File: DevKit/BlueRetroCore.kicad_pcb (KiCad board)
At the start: 4 copper layers, 85 x 56 mm, 108 parts, among them J1 USB_C_Receptacle_USB2.0, J2 Conn_02x06, J3 Micro_SD_Card, J4 Conn_01x03, J5 DB25_Female_MountingHoles, J6 Conn_02x13, J7 Conn_02x07, Q1 BSS138, Q2 BSS138, Q3 S8050, Q4 S8050, Q5 S8050, SW1 BOOT, SW2 EN, U1 ESP32-WROOM, U10 TPD6F003, U11 TPD6F003, U12 TPD6F003, U13 TPD6F003, U2 FT2232HL, U3 STL6N3LLH6, U4 TCPP01-M12, U5 M93C46, U6 ECMF02-2AMX6, U7 TPD6F003, U8 AP7361C-33E, U9 AP7361C-33E, Y1 12MHz

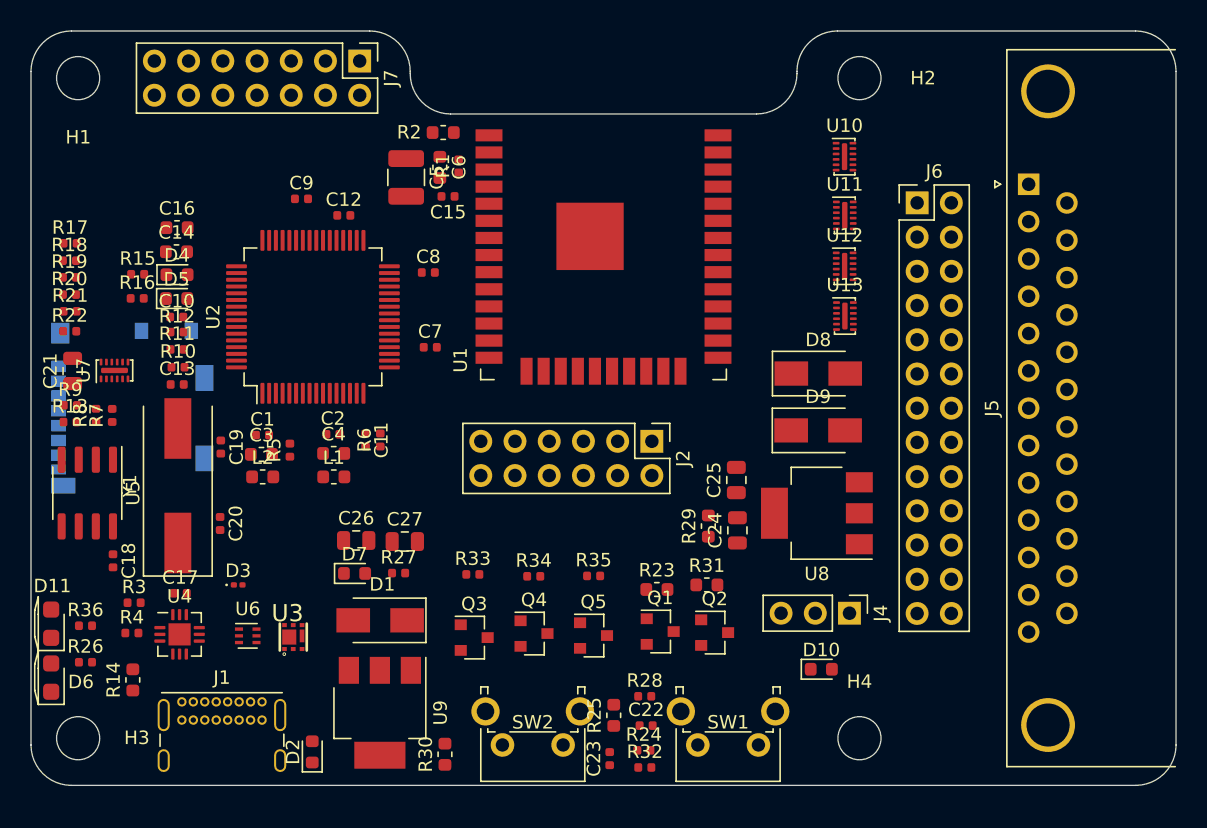
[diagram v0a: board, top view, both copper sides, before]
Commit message: PCB routing
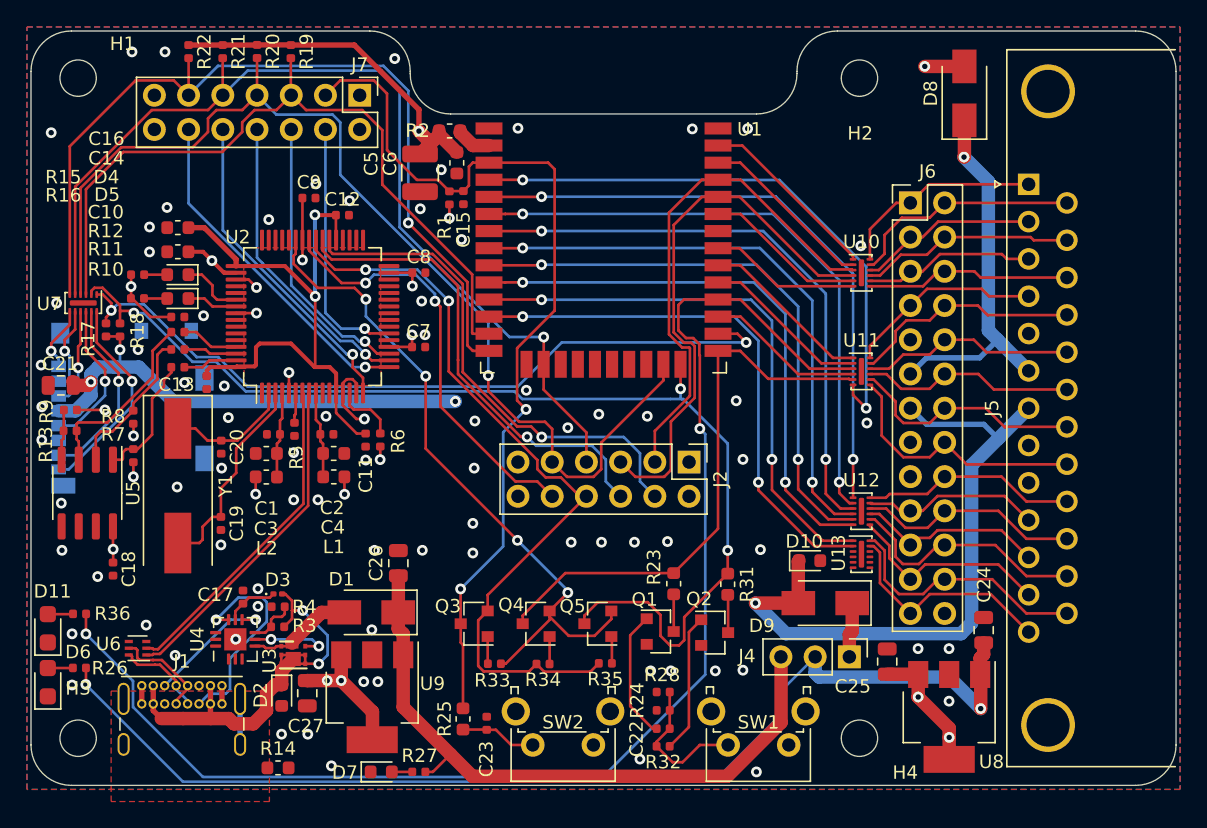
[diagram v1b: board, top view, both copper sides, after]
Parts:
- removed R29, R30: 0, BlueRetro:R_0603_1608Metric
- H1, H2, H3, H4: footprint BlueRetro:MountingHole_3.2mm_M3 -> BlueRetro:MountingHole_2.7mm_M2.5
- U1: value ESP32-WROOM -> ESP32-WROOM-32E
- U8, U9: footprint BlueRetro:SOT-223-3_TabPin2 -> BlueRetro:SOT-223-3_TabPin3
- moved R19 23.5 mm to (-23.2, -26.5), turned to 270 degrees
- moved D8 23.5 mm to (26.8, -23.4), turned to 90 degrees
- moved R20 22.8 mm to (-25.7, -26.5), turned to 270 degrees
- moved R22 22.6 mm to (-30.8, -26.5), turned to 270 degrees
- moved R21 22.4 mm to (-28.3, -26.5), turned to 270 degrees
- moved C24 19.7 mm to (28.2, 16.5)
- moved U12 18.2 mm to (19.1, 7.65)
- moved U8 18.0 mm to (25.7, 22.9), turned to 270 degrees
- moved U13 17.7 mm to (19.1, 10.8)
- moved C25 17.5 mm to (21.1, 18.8)
- moved D7 14.9 mm to (-16.5, 27.0)
- moved R27 14.8 mm to (-13.7, 27.0), turned to 180 degrees
- moved C27 13.4 mm to (-22.0, 21.2), turned to 270 degrees
- moved D9 12.8 mm to (16.5, 14.5), turned to 180 degrees
- moved R14 12.6 mm to (-24.2, 26.7), turned to 0 degrees
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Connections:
- net Net-(J1-PadA6) renamed /USB_C_P
- net Net-(J1-PadA7) renamed /USB_C_N
- net Net-(U2-Pad7) renamed /USB_N
- net Net-(U2-Pad8) renamed /USB_P
- J1 pad A8: (no net) -> Net-(J1-PadA8)
- J1 pad B8: (no net) -> Net-(J1-PadB8)
- J3 pad 10: (no net) -> Net-(J3-Pad10)
- J3 pad 9: (no net) -> Net-(J3-Pad9)
- J5 pad 1: /IO19_C -> /IO23_C
- J5 pad 10: /IO32_C -> /I34_C
- J5 pad 11: /IO33_C -> /IO32_C
- J5 pad 12: /I34_C -> /IO25_C
- J5 pad 13: /I35_C -> /IO27_C
- J5 pad 14: /IO0_C -> /IO22_C
- J5 pad 15: /IO1_C -> /IO3_C
- J5 pad 16: /IO3_C -> /IO19_C
- J5 pad 18: /IO16_C -> /IO17_C
- J5 pad 19: /IO17_C -> /IO16_C
- J5 pad 2: /IO21_C -> /IO1_C
- J5 pad 20: /IO18_C -> /IO0_C
- J5 pad 21: /IO23_C -> /I36_C
- J5 pad 22: /IO26_C -> /I39_C
- J5 pad 23: /IO27_C -> /I35_C
- J5 pad 24: /I36_C -> /IO33_C
- J5 pad 25: /I39_C -> /IO26_C
- J5 pad 3: /IO22_C -> /IO21_C
- J5 pad 4: /IO25_C -> /IO18_C
- J6 pad 1: /IO19_C -> /IO23_C
- J6 pad 10: /IO32_C -> /I34_C
- J6 pad 11: /IO33_C -> /IO32_C
- J6 pad 12: /I34_C -> /IO25_C
- J6 pad 13: /I35_C -> /IO27_C
- J6 pad 14: /IO0_C -> /IO22_C
- J6 pad 15: /IO1_C -> /IO3_C
- J6 pad 16: /IO3_C -> /IO19_C
- J6 pad 18: /IO16_C -> /IO17_C
- J6 pad 19: /IO17_C -> /IO16_C
- J6 pad 2: /IO21_C -> /IO1_C
- J6 pad 20: /IO18_C -> /IO0_C
- J6 pad 21: /IO23_C -> /I36_C
- J6 pad 22: /IO26_C -> /I39_C
- J6 pad 23: /IO27_C -> /I35_C
- J6 pad 24: /I36_C -> /IO33_C
- J6 pad 25: /I39_C -> /IO26_C
- J6 pad 3: /IO22_C -> /IO21_C
- J6 pad 4: /IO25_C -> /IO18_C
- J7 pad 10: /TMS -> /TCK
- J7 pad 11: /EN -> /IO12
- J7 pad 12: /nTRST -> /TDI
- J7 pad 3: /IO13 -> /EN
- J7 pad 4: /TCK -> /nTRST
- J7 pad 5: /IO12 -> /IO14
- J7 pad 6: /TDI -> /TMS
- J7 pad 9: /IO14 -> /IO13
- U1 pad 17: (no net) -> Net-(U1-Pad17)
- U1 pad 18: (no net) -> Net-(U1-Pad18)
- U1 pad 19: (no net) -> Net-(U1-Pad19)
- U1 pad 20: (no net) -> Net-(U1-Pad20)
- U1 pad 21: (no net) -> Net-(U1-Pad21)
- U1 pad 22: (no net) -> Net-(U1-Pad22)
- U1 pad 32: (no net) -> Net-(U1-Pad32)
- U10 pad 1: /IO19 -> /IO23
- U10 pad 10: /IO21_C -> /IO1_C
- U10 pad 11: /IO0_C -> /IO22_C
- U10 pad 12: /IO19_C -> /IO23_C
- U10 pad 2: /IO0 -> /IO22
- U10 pad 3: /IO21 -> /IO1
- U10 pad 4: /IO1 -> /IO3
- U10 pad 5: /IO22 -> /IO21
- U10 pad 6: /IO3 -> /IO19
- U10 pad 7: /IO3_C -> /IO19_C
- U10 pad 8: /IO22_C -> /IO21_C
- U10 pad 9: /IO1_C -> /IO3_C
- U11 pad 1: /IO25 -> /IO18
- U11 pad 10: /IO16_C -> /IO17_C
- U11 pad 12: /IO25_C -> /IO18_C
- U11 pad 3: /IO16 -> /IO17
- U11 pad 4: /IO17 -> /IO16
- U11 pad 5: /IO18 -> /IO0
- U11 pad 6: /IO23 -> /I36
- U11 pad 7: /IO23_C -> /I36_C
- U11 pad 8: /IO18_C -> /IO0_C
- U11 pad 9: /IO17_C -> /IO16_C
- U12 pad 1: /IO26 -> /I39
- U12 pad 10: /IO27_C -> /I35_C
- U12 pad 11: /IO32_C -> /I34_C
- U12 pad 12: /IO26_C -> /I39_C
- U12 pad 2: /IO32 -> /I34
- U12 pad 3: /IO27 -> /I35
- U12 pad 4: /IO33 -> /IO32
- U12 pad 5: /I36 -> /IO33
- U12 pad 6: /I34 -> /IO25
- U12 pad 7: /I34_C -> /IO25_C
- U12 pad 8: /I36_C -> /IO33_C
- U12 pad 9: /IO33_C -> /IO32_C
- U13 pad 1: /I39 -> /IO26
- U13 pad 10: (no net) -> Net-(U13-Pad10)
- U13 pad 11: /I35_C -> /IO27_C
- U13 pad 12: /I39_C -> /IO26_C
- U13 pad 2: /I35 -> /IO27
- U13 pad 3: (no net) -> Net-(U13-Pad3)
- U13 pad 4: (no net) -> Net-(U13-Pad4)
- U13 pad 5: (no net) -> Net-(U13-Pad5)
- U13 pad 6: (no net) -> Net-(U13-Pad6)
- U13 pad 7: (no net) -> Net-(U13-Pad7)
- U13 pad 8: (no net) -> Net-(U13-Pad8)
- U13 pad 9: (no net) -> Net-(U13-Pad9)
- U2 pad 21: (no net) -> Net-(U2-Pad21)
- U2 pad 23: (no net) -> Net-(U2-Pad23)
- U2 pad 24: (no net) -> Net-(U2-Pad24)
- U2 pad 26: (no net) -> Net-(U2-Pad26)
- U2 pad 27: (no net) -> Net-(U2-Pad27)
- U2 pad 28: (no net) -> Net-(U2-Pad28)
- U2 pad 29: (no net) -> Net-(U2-Pad29)
- U2 pad 30: (no net) -> Net-(U2-Pad30)
- U2 pad 32: (no net) -> Net-(U2-Pad32)
- U2 pad 33: (no net) -> Net-(U2-Pad33)
- U2 pad 34: (no net) -> Net-(U2-Pad34)
- U2 pad 36: (no net) -> Net-(U2-Pad36)
- U2 pad 44: (no net) -> Net-(U2-Pad44)
- U2 pad 45: (no net) -> Net-(U2-Pad45)
- U2 pad 46: (no net) -> Net-(U2-Pad46)
- U2 pad 48: (no net) -> Net-(U2-Pad48)
- U2 pad 52: (no net) -> Net-(U2-Pad52)
- U2 pad 53: (no net) -> Net-(U2-Pad53)
- U2 pad 57: (no net) -> Net-(U2-Pad57)
- U2 pad 58: (no net) -> Net-(U2-Pad58)
- U2 pad 59: (no net) -> Net-(U2-Pad59)
- U2 pad 60: (no net) -> Net-(U2-Pad60)
- U3 pad 1: Net-(D1-Pad2) -> Net-(D2-Pad1)
- U3 pad 2: Net-(D1-Pad2) -> Net-(D2-Pad1)
- U3 pad 3: Net-(D1-Pad2) -> Net-(U3-Pad3)
- U3 pad 4: Net-(U3-Pad4) -> Net-(D1-Pad2)
- U3 pad 8: Net-(D2-Pad1) -> Net-(D1-Pad2)
- U4 pad 5: Net-(U3-Pad4) -> Net-(U3-Pad3)
- U5 pad 6: (no net) -> Net-(U5-Pad6)
- U5 pad 7: (no net) -> Net-(U5-Pad7)
- U6 pad 4: (no net) -> Net-(U6-Pad4)
- U7 pad 1: /IO12 -> /IO4
- U7 pad 10: Net-(J3-Pad3) -> Net-(J3-Pad5)
- U7 pad 11: Net-(J3-Pad2) -> Net-(J3-Pad7)
- U7 pad 12: Net-(J3-Pad1) -> Net-(J3-Pad8)
- U7 pad 2: /IO13 -> /IO2
- U7 pad 3: /IO15 -> /IO14
- U7 pad 4: /IO14 -> /IO15
- U7 pad 5: /IO2 -> /IO13
- U7 pad 6: /IO4 -> /IO12
- U7 pad 7: Net-(J3-Pad8) -> Net-(J3-Pad1)
- U7 pad 8: Net-(J3-Pad7) -> Net-(J3-Pad2)
- U7 pad 9: Net-(J3-Pad5) -> Net-(J3-Pad3)
- U8 pad 2: Net-(R29-Pad1) -> GND
- U9 pad 2: Net-(R30-Pad1) -> GND
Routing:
- net /IO17: track 0.00 -> 100.0 mm, vias 0 -> 2
- net /IO2: track 0.00 -> 82.9 mm, vias 0 -> 3
- net +5V: track 0.00 -> 82.9 mm, vias 0 -> 2
- net /IO15: track 0.00 -> 81.1 mm, vias 0 -> 1
- net +3V3: track 0.00 -> 77.3 mm, vias 0 -> 8
- net /IO13: track 0.00 -> 73.9 mm, vias 0 -> 1
- net /EN: track 0.00 -> 68.8 mm, vias 0 -> 2
- net /IO12: track 0.00 -> 65.5 mm, vias 0 -> 1
- net /nRTS: track 0.00 -> 57.6 mm, vias 0 -> 2
- net /IO4: track 0.00 -> 56.6 mm, vias 0 -> 2
- net /IO14: track 0.00 -> 56.1 mm
- net /nDTR: track 0.00 -> 50.5 mm, vias 0 -> 4
- net VBUS: track 0.00 -> 49.0 mm
- net /VIN_C: track 0.00 -> 48.8 mm, vias 0 -> 1
- net /I39: track 0.00 -> 46.0 mm, vias 0 -> 2
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- added copper zone on F.Cu, net +1V8
- added copper zone on In2.Cu, net +3V3
- added copper zone on In2.Cu, net +3V3_USB
- added copper zone on B.Cu, net GND
- added copper zone on F.Cu, net GND
- added copper zone on In1.Cu, net GND
- added copper zone on F.Cu, net Net-(J1-PadS1)
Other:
- net class Default: clearance 0.2 -> 0.15; trace_width 0.25 -> 0.2
- rule trace_clearance: 0.2 -> 0.15
- rule trace_min: 0.2 -> 0.15
